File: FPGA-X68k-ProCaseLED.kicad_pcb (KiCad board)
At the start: 2 copper layers, 80 x 36 mm, 47 parts, among them J1 Conn_01x05_Male, SW1 SW_DIP_x04, U1 TLC59116IPWR

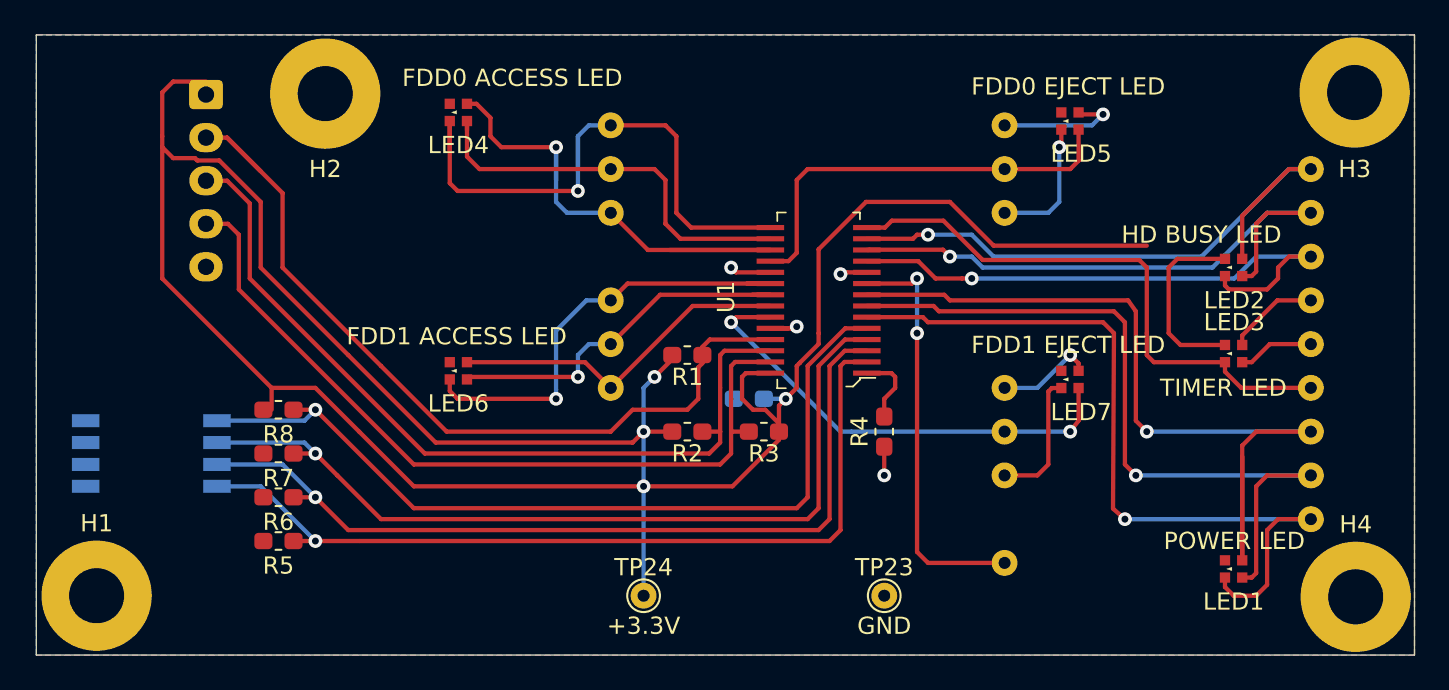
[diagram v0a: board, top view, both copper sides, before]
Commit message: First version
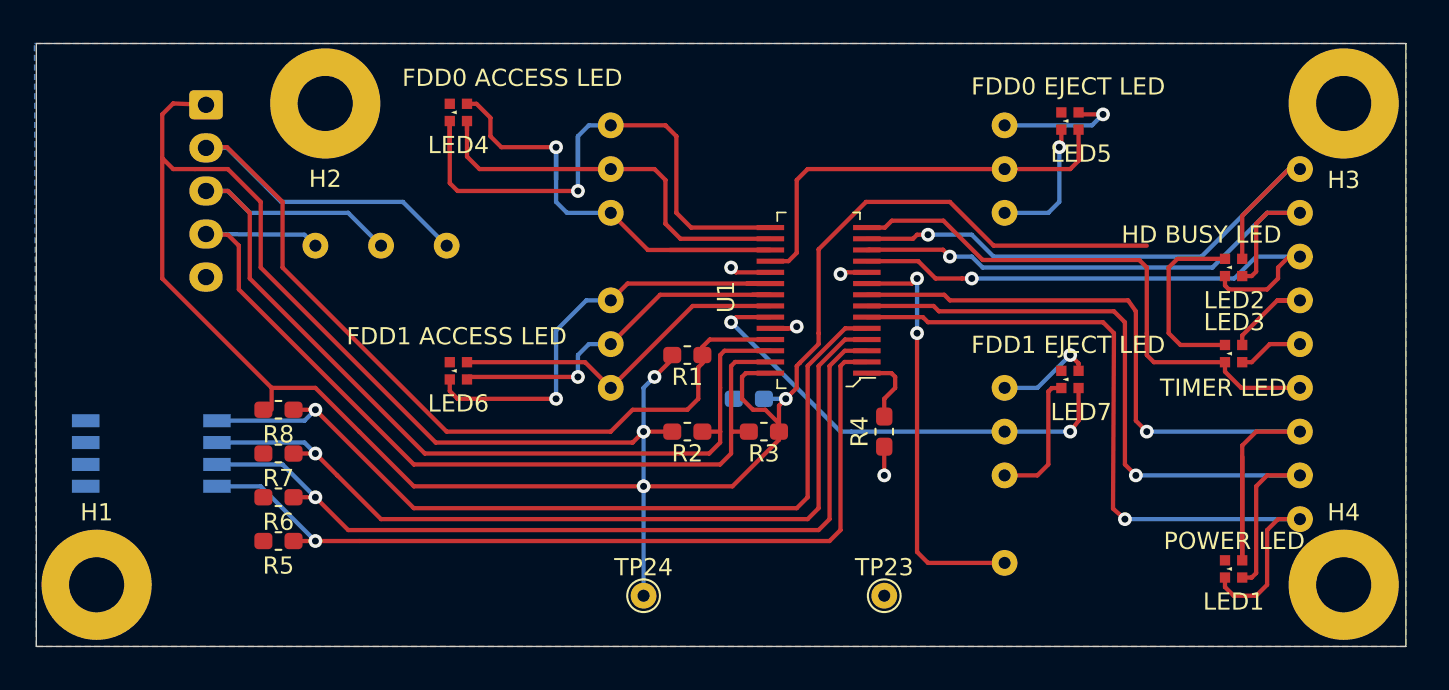
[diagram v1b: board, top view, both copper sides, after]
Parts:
- added TP25: RESET, TestPoint:TestPoint_THTPad_D1.5mm_Drill0.7mm, B.Cu at (83.8, 102.2)
- added TP26: SCL, TestPoint:TestPoint_THTPad_D1.5mm_Drill0.7mm, B.Cu at (80.0, 102.2)
- added TP27: SDA, TestPoint:TestPoint_THTPad_D1.5mm_Drill0.7mm, B.Cu at (76.2, 102.2)
- TP24: value +3.3V -> +3V3
- moved H4 0.99 mm to (135.9, 121.9)
- moved H3 0.90 mm to (135.9, 94.0)
- moved TP10 0.64 mm to (133.3, 105.4)
- moved TP2 0.64 mm to (133.3, 118.1)
- moved TP3 0.64 mm to (133.3, 115.6)
- moved TP4 0.64 mm to (133.3, 113.0)
- moved TP5 0.64 mm to (133.3, 102.9)
- moved TP6 0.64 mm to (133.3, 100.3)
- moved TP7 0.64 mm to (133.3, 97.8)
- moved TP8 0.64 mm to (133.3, 110.5)
- moved TP9 0.64 mm to (133.3, 108.0)
- moved H1 0.64 mm to (63.5, 121.9)
- moved J1 0.59 mm to (69.8, 94.1)
- moved H2 0.57 mm to (76.8, 94.0)
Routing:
- net /RESET: track 49.0 -> 62.0 mm
- net /SCL: track 48.3 -> 59.3 mm
- net /SDA: track 46.9 -> 52.9 mm
- net +3V3: track 162.2 -> 160.7 mm
- net /TIMER_LED_B: track 5.38 -> 6.69 mm
- net /POWER_LED_B: track 49.9 -> 48.6 mm
- net /HD_BUSY_LED_G: track 34.7 -> 33.4 mm
- net /TIMER_LED_R: track 33.3 -> 32.6 mm
- net /TIMER_LED_G: track 4.42 -> 3.78 mm
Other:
- board size 80 x 36 mm -> 79.5 x 35 mm
